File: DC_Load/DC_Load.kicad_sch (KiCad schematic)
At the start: 90 parts, among them J1 Conn_01x02_Pin, J2 Conn_01x02_Pin, J3 Conn_01x04_Pin, Q11 BC547, Q9 NMOS, SW1 MENU, SW2 START, SW3 STOP, SW4 Enter, SW5 Back, SW6 F1, SW8 RotaryEncoder, U1 MCP6034, U10 MCP6001-OT, U11 AT90CAN64-16A, U12 TL431LP, U13 MCP4822, U14 MCP4822, U15 MCP3422, U2 MCP2551-I-SN, U3 MCP4822, U4 NX3L4051PW_118, U5 MCP6034, U6 MCP4822, U7 MCP6034, U8 MCP6034, U9 L7805, Y1 Crystal

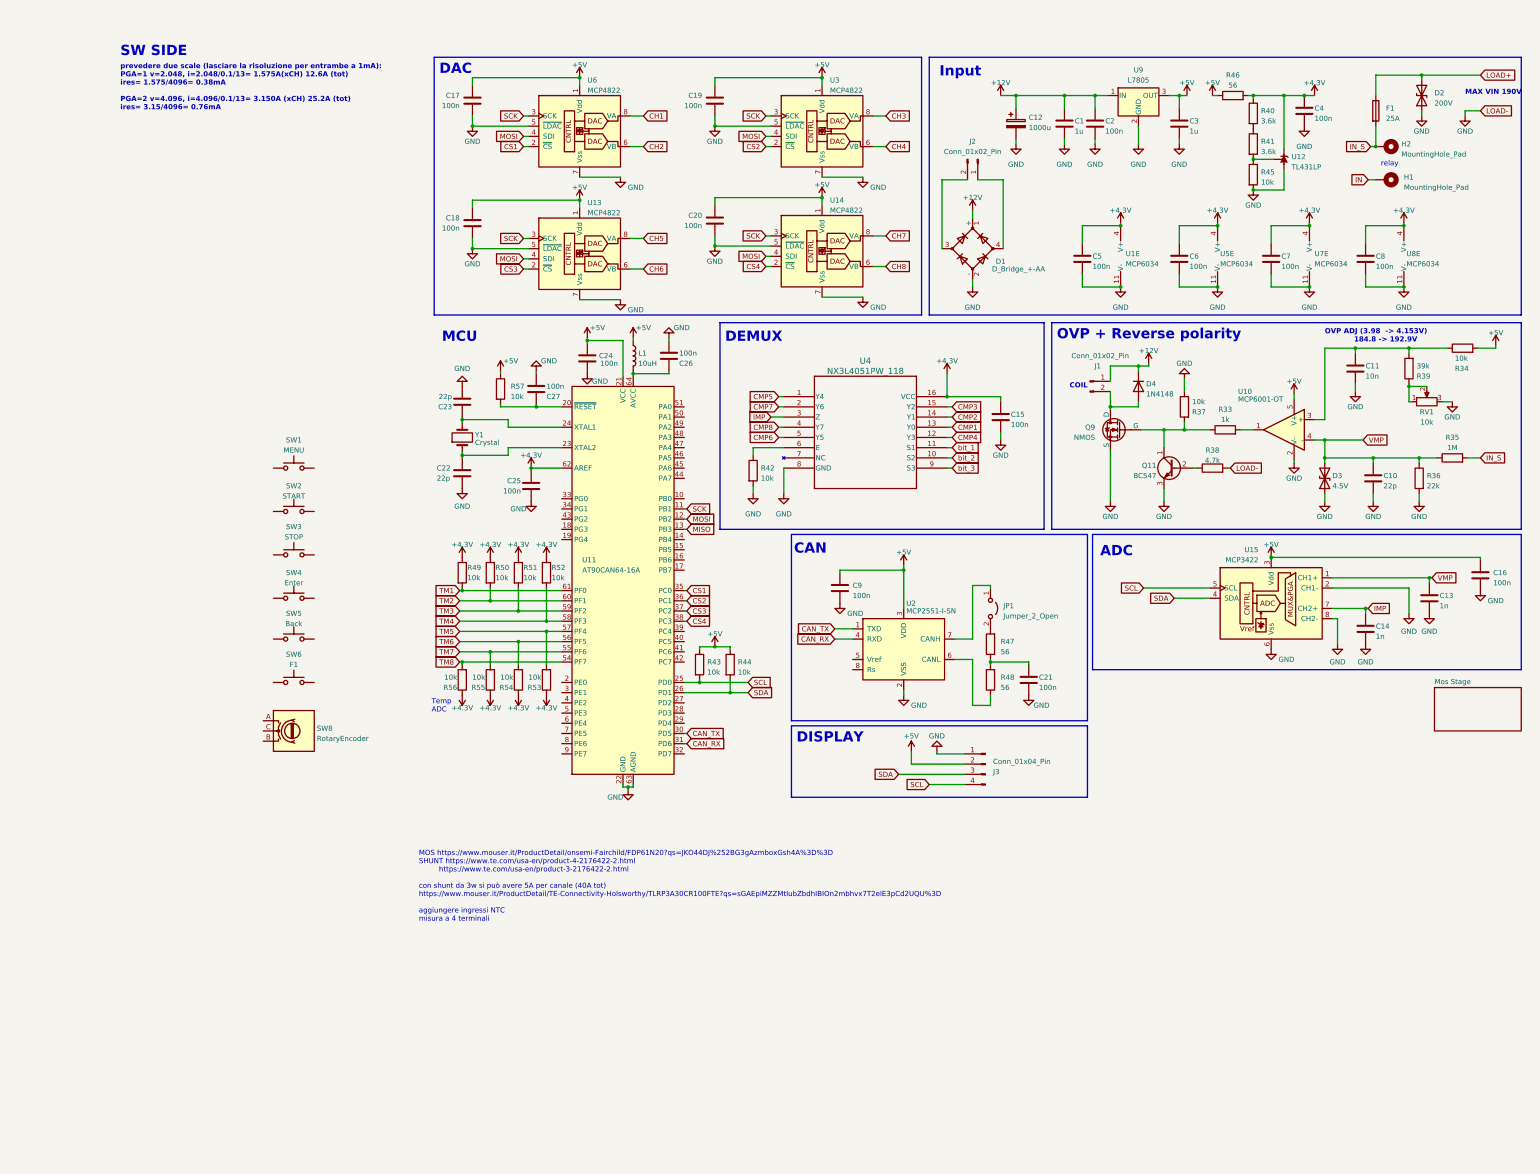
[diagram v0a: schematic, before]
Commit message: Add files via upload
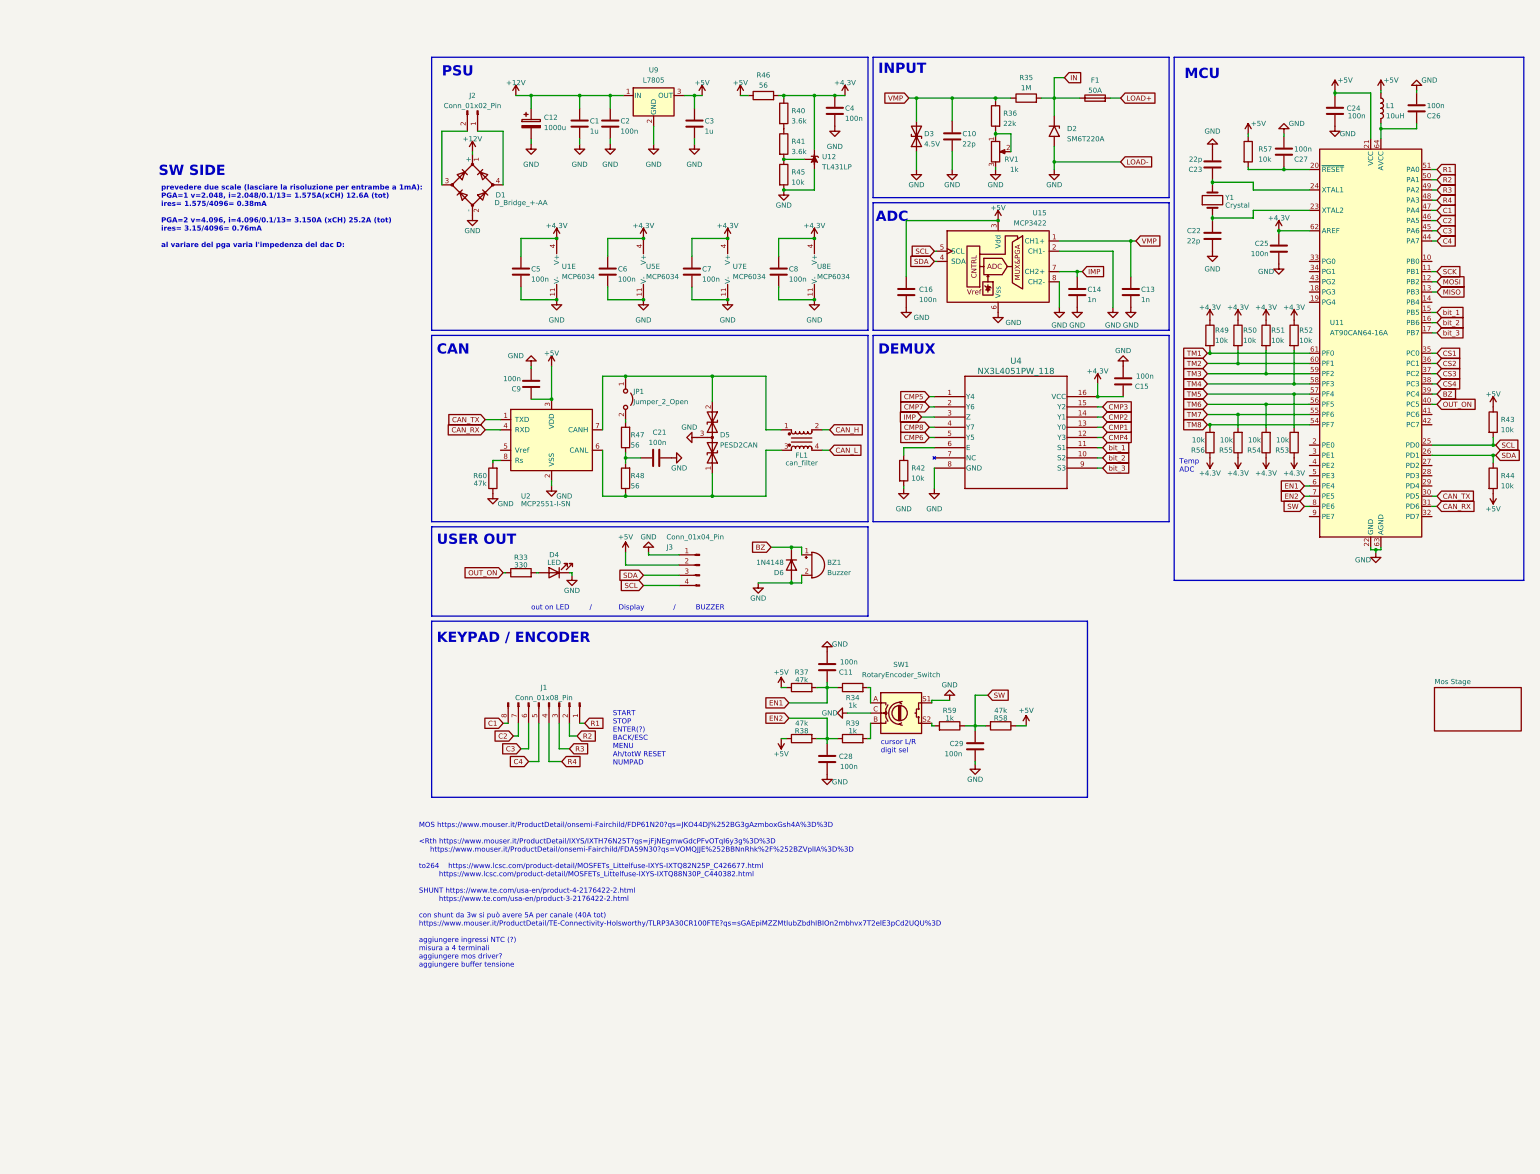
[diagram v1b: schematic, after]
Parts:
- removed C17, C18, C19, C20: 100n, symbol Device:C
- removed D2: 200V, symbol Device:D_TVS
- removed D4: 1N4148, Diode_THT:D_DO-35_SOD27_P7.62mm_Horizontal, symbol Diode:1N4148
- removed H1, H2: MountingHole_Pad, symbol Mechanical:MountingHole_Pad
- removed J1: Conn_01x02_Pin, symbol Connector:Conn_01x02_Pin
- removed Q11: BC547, Package_TO_SOT_THT:TO-92_Inline, symbol Transistor_BJT:BC547
- removed Q9: NMOS, symbol Simulation_SPICE:NMOS
- removed SW1: MENU, symbol Switch:SW_Push
- removed SW2: START, symbol Switch:SW_Push
- removed SW3: STOP, symbol Switch:SW_Push
- removed SW4: Enter, symbol Switch:SW_Push
- removed SW5: Back, symbol Switch:SW_Push
- removed SW6: F1, symbol Switch:SW_Push
- removed SW8: RotaryEncoder, symbol Device:RotaryEncoder
- removed U10: MCP6001-OT, Package_TO_SOT_SMD:SOT-23-5, symbol Amplifier_Operational:MCP6001-OT
- removed U13, U14, U3, U6: MCP4822, symbol Analog_DAC:MCP4822
- added BZ1: Buzzer, symbol Device:Buzzer
- added C28, C29: 100n, symbol Device:C
- added D2: SM6T220A, Diode_SMD:D_SMB, symbol Diode:SM6T220A
- added D4: LED, symbol Device:LED
- added D5: PESD2CAN, symbol Device:D_TVS_Dual_AAC
- added D6: 1N4148, Diode_THT:D_DO-35_SOD27_P7.62mm_Horizontal, symbol Diode:1N4148
- added FL1: can_filter, Inductor_THT:Choke_Schaffner_RN102-04-14.0x14.0mm, symbol Filter:Choke_Schaffner_RN102-0.3-02-12M
- added J1: Conn_01x08_Pin, symbol Connector:Conn_01x08_Pin
- added R58, R60: 47k, symbol Device:R
- added R59: 1k, symbol Device:R
- added SW1: RotaryEncoder_Switch, symbol Device:RotaryEncoder_Switch
- C11: value 10n -> 100n
- F1: value 25A -> 50A
- R33: value 1k -> 330
- R34, RV1: value 10k -> 1k
- R37: value 10k -> 47k
- R38: value 4.7k -> 47k
- R39: value 39k -> 1k
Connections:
- net +5V: now also R37.1, R38.1, R44.2, R58.1; no longer R34.2, R44.1
- net GND: now also BZ1.2 (+), C28.2, C29.2, D2.2 (A2), D4.1 (K), D5.3 (common), D6.2 (A), R60.1, SW1.C, SW1.S1; no longer R36.2, R37.1, R38.2
- net IN: now also F1.1, R35.2, D2.1 (A1)
- net LOAD+: now also F1.2; no longer F1.1
- net SDA: now also R44.1; no longer R44.2
- net bit_1: now also U11.15 (PB5)
- net bit_2: now also U11.16 (PB6)
- net bit_3: now also U11.17 (PB7)
- net EN1: now reaches R37.2
- net EN1: now also C11.1, R34.1, U11.6 (PE4); no longer R33.1
- net at R48.1, U2.6 (CANL): now also D5.1 (A1), FL1.3
- net at JP1.1 (A), U2.7 (CANH): now also D5.2 (A2), FL1.1
- net at U2.8 (Rs): now also R60.2
- net at R33.2: now also D4.2 (A)
- net at RV1.1, RV1.2: now also R36.2; no longer R39.1
- net BZ: now reaches U11.39 (PC4)
- net BZ: now also BZ1.1 (-), D6.1 (K)
- net OUT_ON: now reaches U11.40 (PC5)
- net OUT_ON: now also R33.1
- net C4: now reaches U11.44 (PA7)
- net C4: now also J1.5 (Pin_5)
- net C3: now reaches U11.45 (PA6)
- net C3: now also J1.6 (Pin_6)
- net C2: now reaches U11.46 (PA5)
- net C2: now also J1.7 (Pin_7)
- net C1: now reaches U11.47 (PA4)
- net C1: now also J1.8 (Pin_8)
- net R4: now reaches U11.48 (PA3)
- net R4: now also J1.4 (Pin_4)
- net R3: now reaches U11.49 (PA2)
- net R3: now also J1.3 (Pin_3)
- net R2: now reaches U11.50 (PA1)
- net R2: now also J1.2 (Pin_2)
- net R1: now reaches U11.51 (PA0)
- net R1: now also J1.1 (Pin_1)
- net EN2: now reaches U11.7 (PE5)
- net EN2: now also R38.2, R39.1, C28.1
- net SW: now reaches U11.8 (PE6)
- net SW: now also C29.1, R58.2, R59.1
- removed net IN_S: F1.2, R35.2
- new net: R39.2, SW1.B
- new net: R59.2, SW1.S2
- new net: R34.2, SW1.A
- new net CAN_H: FL1.2
- new net CAN_L: FL1.4
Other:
- note added: "INPUT"
- note added: "KEYPAD / ENCODER"
- note added: "MOS https://www.mouser.it/ProductDetail/onsemi-Fairchild/FDP61N20?qs=JKO44DJ%252BG3gAzmboxGsh4A%3D%3D <Rth https://www.mouser.it/ProductDetail/IXYS/IXTH76N25T?qs=jFjNEgmwGdcPFvOTql6y3g%3D%3D https://www.mouser.it/ProductDetail/onsemi-Fairchild/FDA59N30?qs=VOMQJJE%252BBNnRhk%2F%252BZVplIA%3D%3D to264 https://www.lcsc.com/product-detail/MOSFETs_Littelfuse-IXYS-IXTQ82N25P_C426677.html https://www.lc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"
- note added: "PSU"
- note added: "START STOP ENTER(?) BACK/ESC MENU Ah/totW RESET NUMPAD"
- note added: "USER OUT"
- note added: "cursor L/R digit sel"
- note added: "out on LED / Display / BUZZER"
- note added: "prevedere due scale (lasciare la risoluzione per entrambe a 1mA): PGA=1 v=2.048, i=2.048/0.1/13= 1.575A(xCH) 12.6A (tot) ires= 1.575/4096= 0.38mA PGA=2 v=4.096, i=4.096/0.1/13= 3.150A (xCH) 25.2A (tot) ires= 3.15/4096= 0.76mA al variare del pga varia l'impedenza del dac D:"
- note removed: "COIL"
- note removed: "DAC"
- note removed: "DISPLAY"
- note removed: "Input"
- note removed: "MAX VIN 190V"
- note removed: "MOS https://www.mouser.it/ProductDetail/onsemi-Fairchild/FDP61N20?qs=JKO44DJ%252BG3gAzmboxGsh4A%3D%3D SHUNT https://www.te.com/usa-en/product-4-2176422-2.html https://www.te.com/usa-en/product-3-2176422-2.html con shunt da 3w si può avere 5A per canale (40A tot) https://www.mouser.it/ProductDetail/TE-Connectivity-Holsworthy/TLRP3A30CR100FTE?qs=sGAEpiMZZMtlubZbdhIBIOn2mbhvx7T2elE3pCd2UQU%3D aggiun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"
- note removed: "OVP + Reverse polarity"
- note removed: "OVP ADJ (3.98 -> 4.153V) 184.8 -> 192.9V"
- note removed: "prevedere due scale (lasciare la risoluzione per entrambe a 1mA): PGA=1 v=2.048, i=2.048/0.1/13= 1.575A(xCH) 12.6A (tot) ires= 1.575/4096= 0.38mA PGA=2 v=4.096, i=4.096/0.1/13= 3.150A (xCH) 25.2A (tot) ires= 3.15/4096= 0.76mA"
- note removed: "relay"
- moved on the sheet: C1, C10, C12, C13, C14, C15, C16, C2, C21, C22, C23, C24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

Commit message: Add files via upload
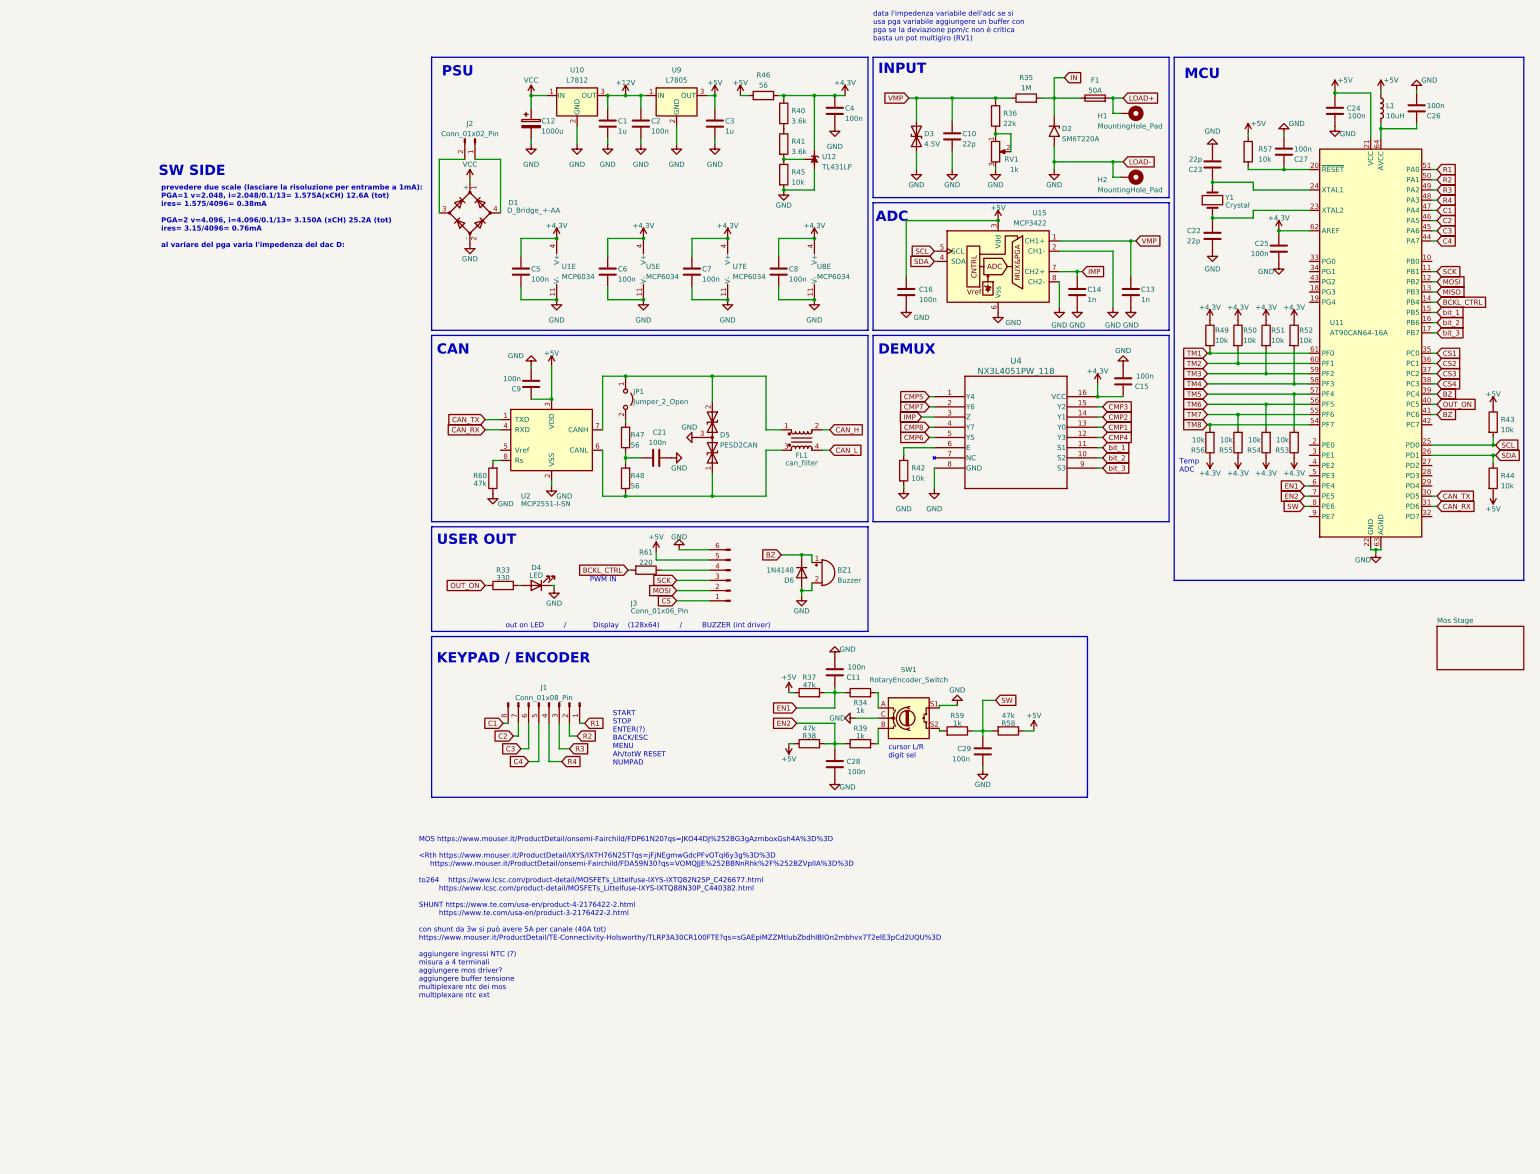
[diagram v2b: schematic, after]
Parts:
- removed J3: Conn_01x04_Pin, symbol Connector:Conn_01x04_Pin
- added H1, H2: MountingHole_Pad, symbol Mechanical:MountingHole_Pad
- added J3: Conn_01x06_Pin, symbol Connector:Conn_01x06_Pin
- added R61: 220, symbol Device:R
- added U10: L7812, symbol Regulator_Linear:L7812
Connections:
- net +12V: now also U10.3 (OUT); no longer C12.1, D1.1 (+)
- net +5V: now also J3.5 (Pin_5)
- net BZ: now also U11.41 (PC6)
- net GND: now also H2.1, J3.6 (Pin_6), U10.2 (GND)
- net LOAD+: now also H1.1
- net MOSI: now also J3.2 (Pin_2)
- net SCK: now also J3.3 (Pin_3)
- net BCKL_CTRL: now reaches U11.14 (PB4)
- net BCKL_CTRL: now also R61.2
- new net: J3.4 (Pin_4), R61.1
- new net CS: J3.1 (Pin_1)
- new net VCC: C12.1, D1.1 (+), U10.1 (IN)
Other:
- note added: "PWM IN"
- note added: "data l'impedenza variabile dell'adc se si usa pga variabile aggiungere un buffer con pga se la deviazione ppm/c non è critica basta un pot multigiro (RV1)"
- note added: "out on LED / Display (128x64) / BUZZER (int driver)"
- note removed: "out on LED / Display / BUZZER"
- moved on the sheet: BZ1, C1, C11, C2, C28, C29, C3, D1, D4, D6, J2, R33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
